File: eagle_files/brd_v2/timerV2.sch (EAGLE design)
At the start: 42 parts, among them IC6 DS1307, U1 ATMEGA328P

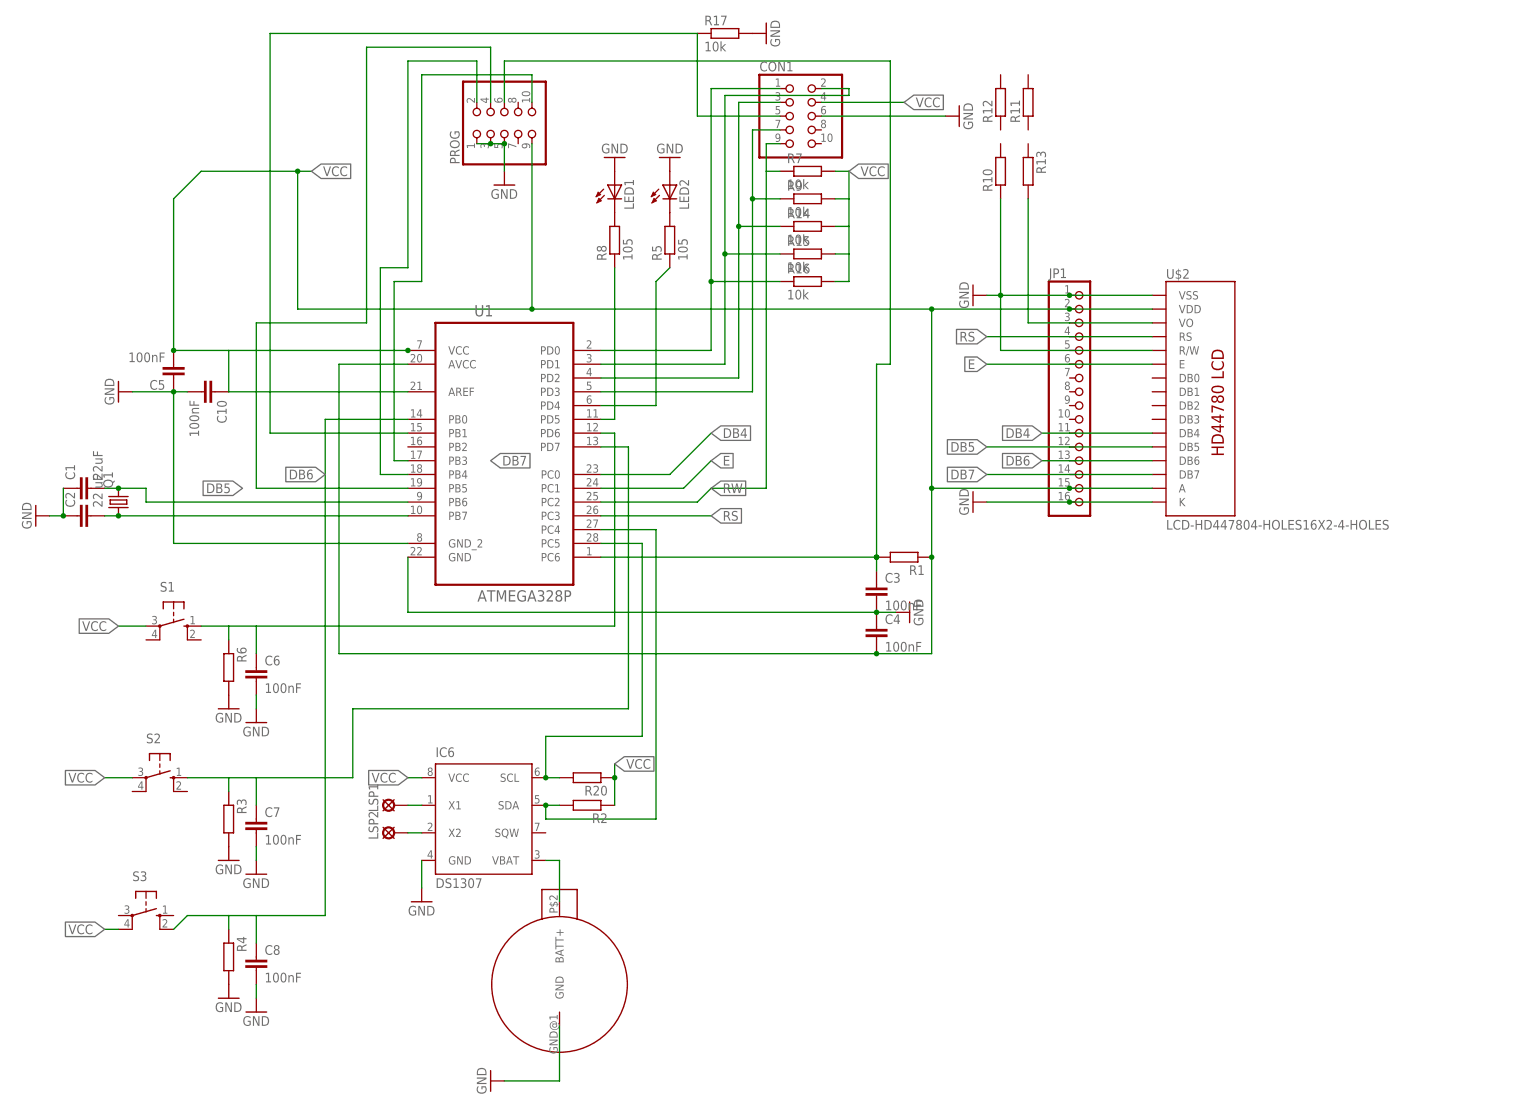
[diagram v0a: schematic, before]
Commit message: Schematic cleaned up
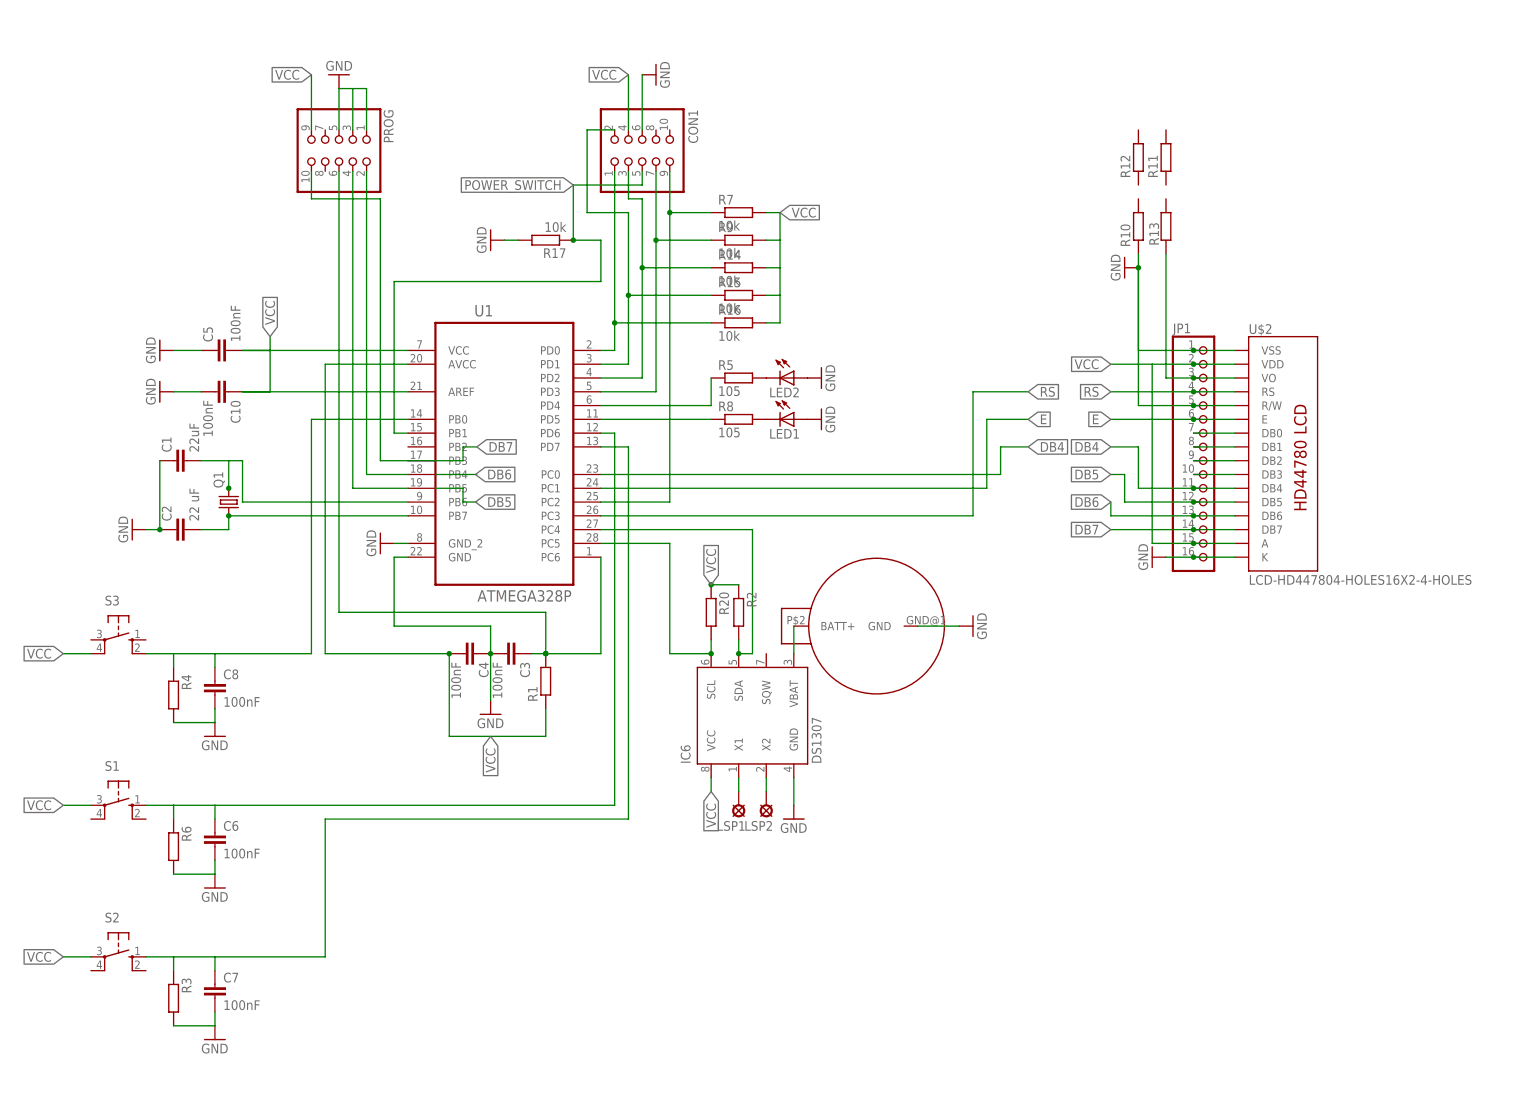
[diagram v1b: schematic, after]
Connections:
- net N$3 renamed POWER_SWITCH
- new net N$10: JP1.7, U$2.DB0
- new net N$16: JP1.8, U$2.DB1
- new net N$18: JP1.9, U$2.DB2
- new net N$19: JP1.10, U$2.DB3
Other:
- moved on the sheet: C1, C10, C2, C3, C4, C5, C6, C7, C8, CON1, IC6, JP1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
